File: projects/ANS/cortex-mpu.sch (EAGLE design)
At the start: 45 parts, among them IC1 LM1117MPX-3.3, U1 AT32UC3B164-AUT, Y1 7A-16

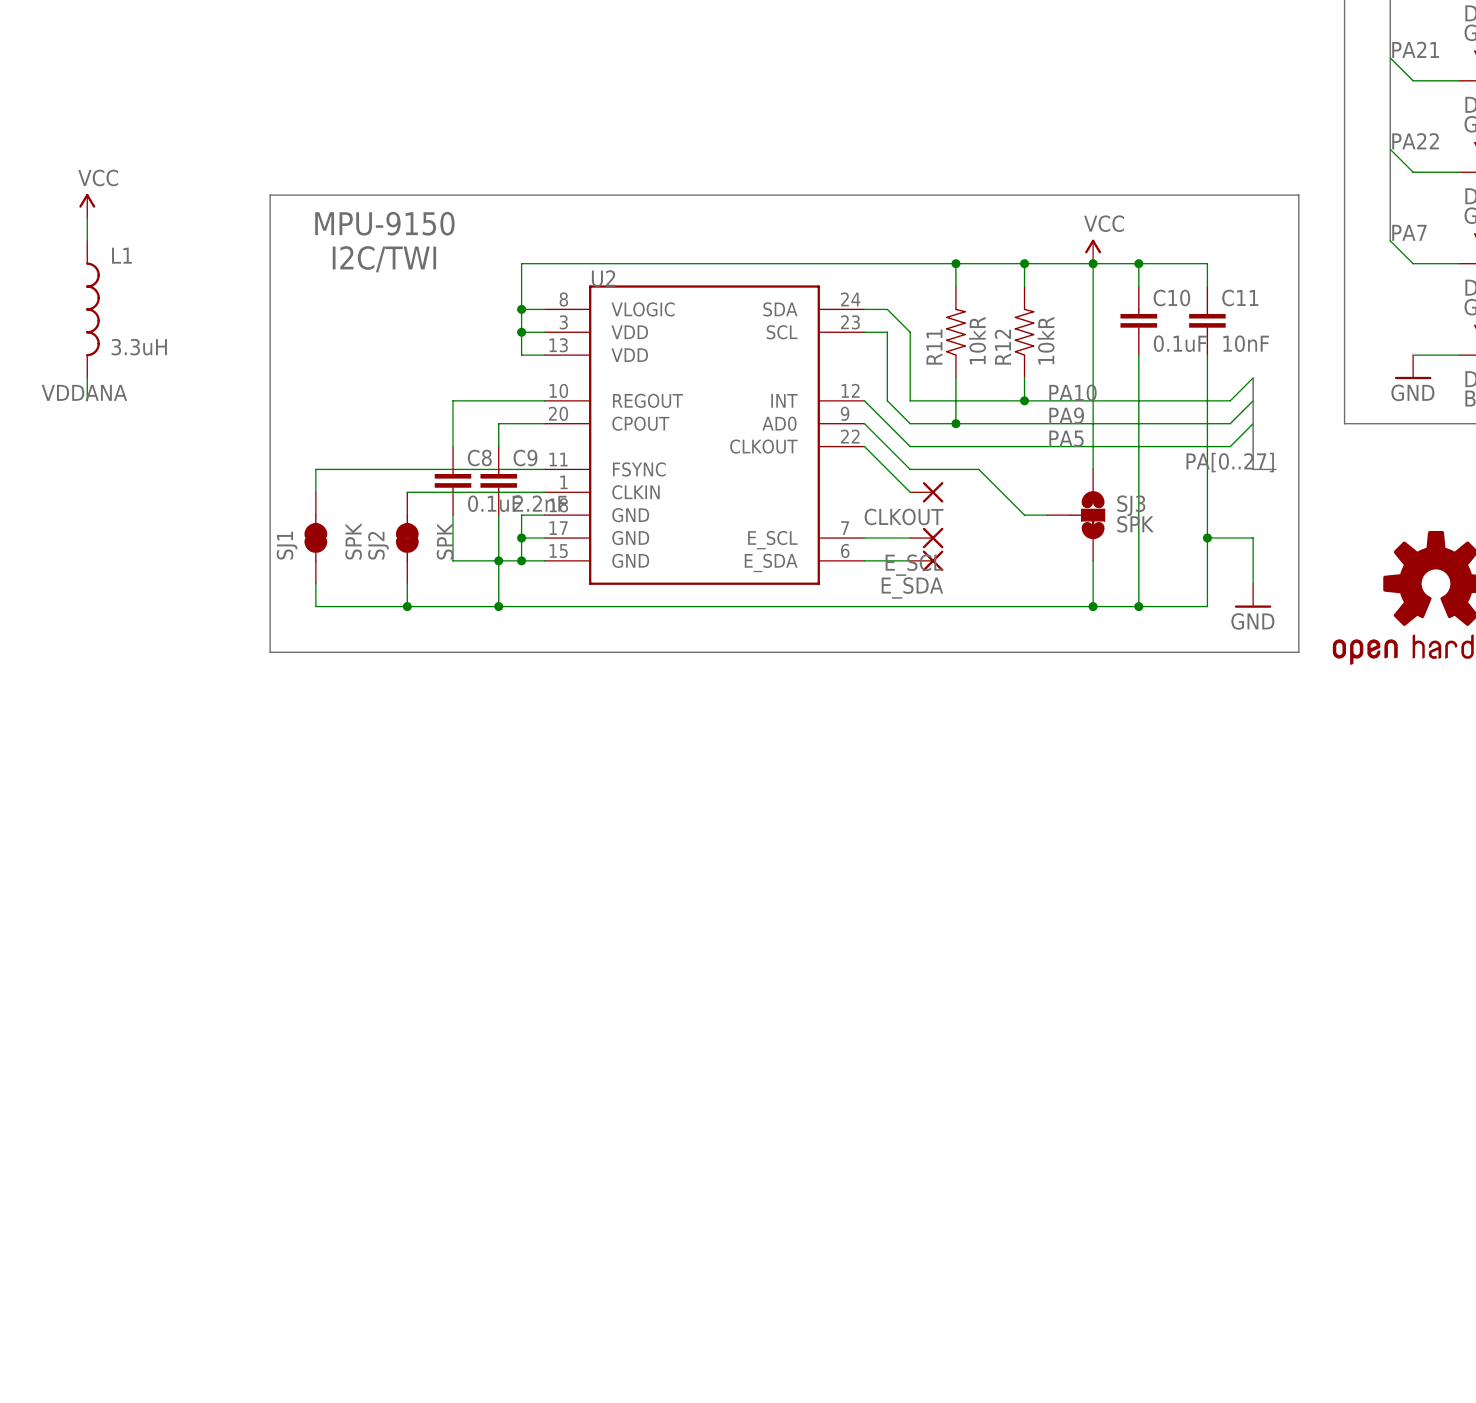
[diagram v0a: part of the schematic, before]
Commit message: Decoupling
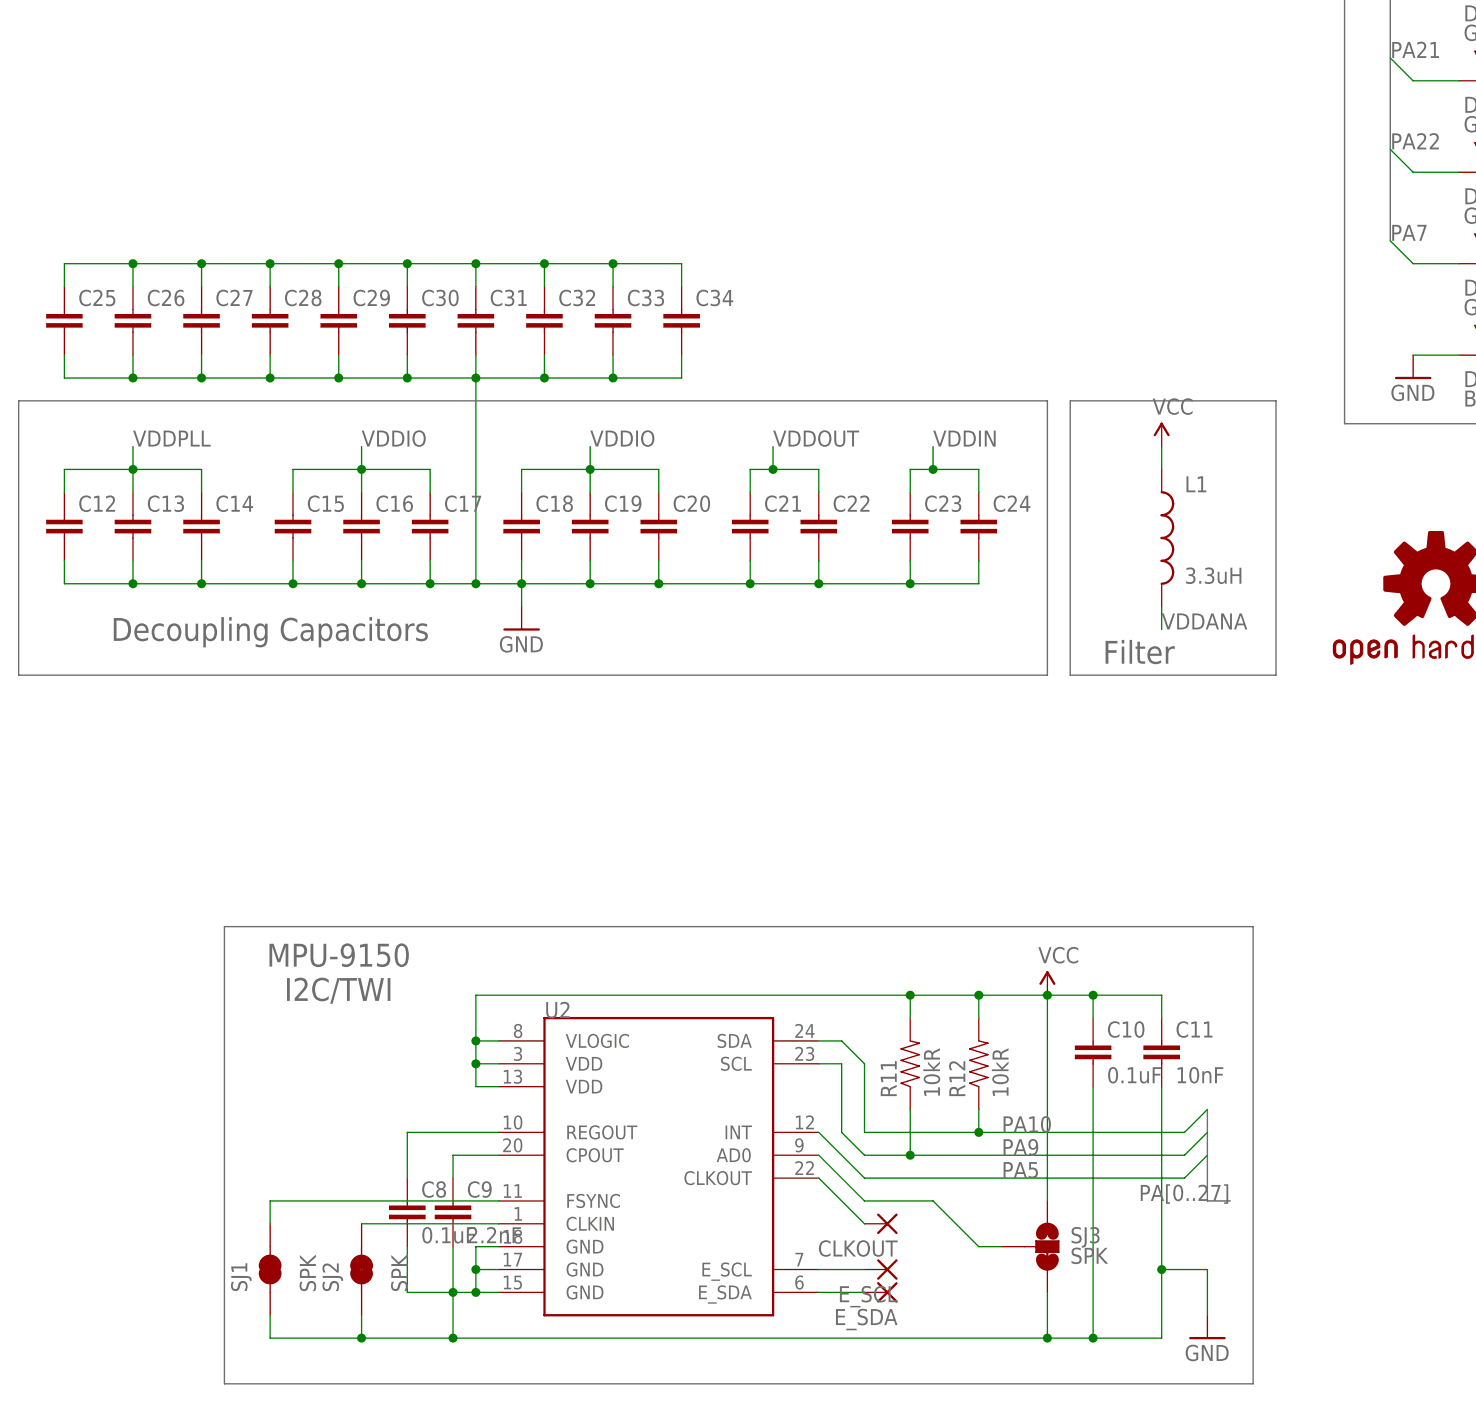
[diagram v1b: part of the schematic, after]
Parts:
- added C12, C13, C14, C15, C16, C17, C18, C19, C20, C21, C22, C23, C24, C25, C26, C27, C28, C29, C30, C31, C32, C33, C34: (no value), SparkFun-Passives:CAP0603-CAP
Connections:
- net GND: now also C12.2, C13.2, C14.2, C15.2, C16.2, C17.2, C18.2, C19.2, C20.2, C21.2, C22.2, C23.2, C24.2, C25.2, C26.2, C27.2, C28.2, C29.2, C30.2, C31.2, C32.2, C33.2, C34.2
- net VDDCORE: now also C25.1, C26.1, C27.1, C28.1, C29.1, C30.1, C31.1, C32.1, C33.1, C34.1
- net VDDIN: now also C23.1, C24.1
- net VDDIO: now also C15.1, C16.1, C17.1, C18.1, C19.1, C20.1
- net VDDOUT: now also C21.1, C22.1
- net VDDPLL: now also C12.1, C13.1, C14.1
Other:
- note added: "Decoupling Capacitors"
- note added: "Filter"
- moved on the sheet: C10, C11, C8, C9, CLKOUT, E_SCL, E_SDA, L1, R11, R12, SJ1, SJ2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

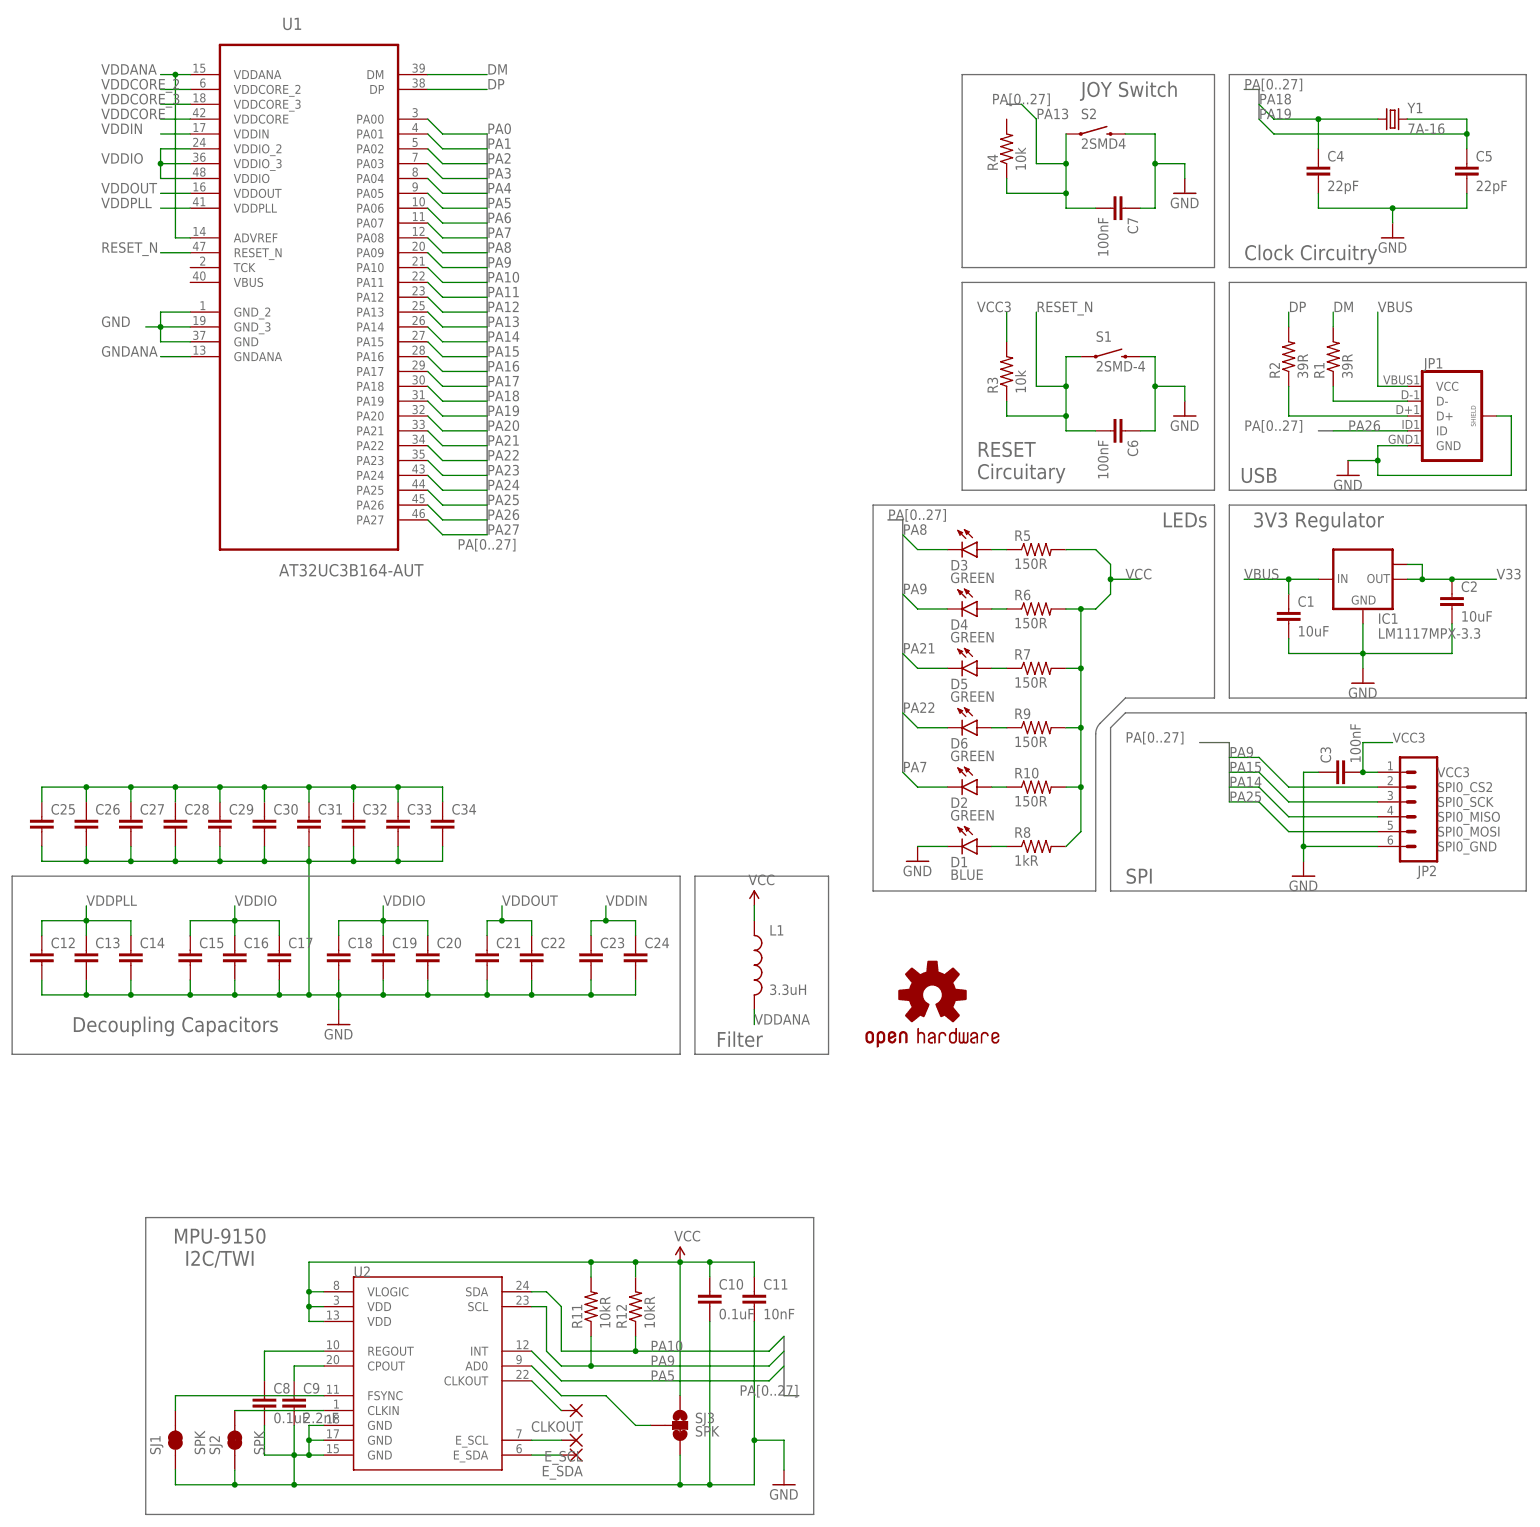
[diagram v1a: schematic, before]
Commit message: Decoupling Capr
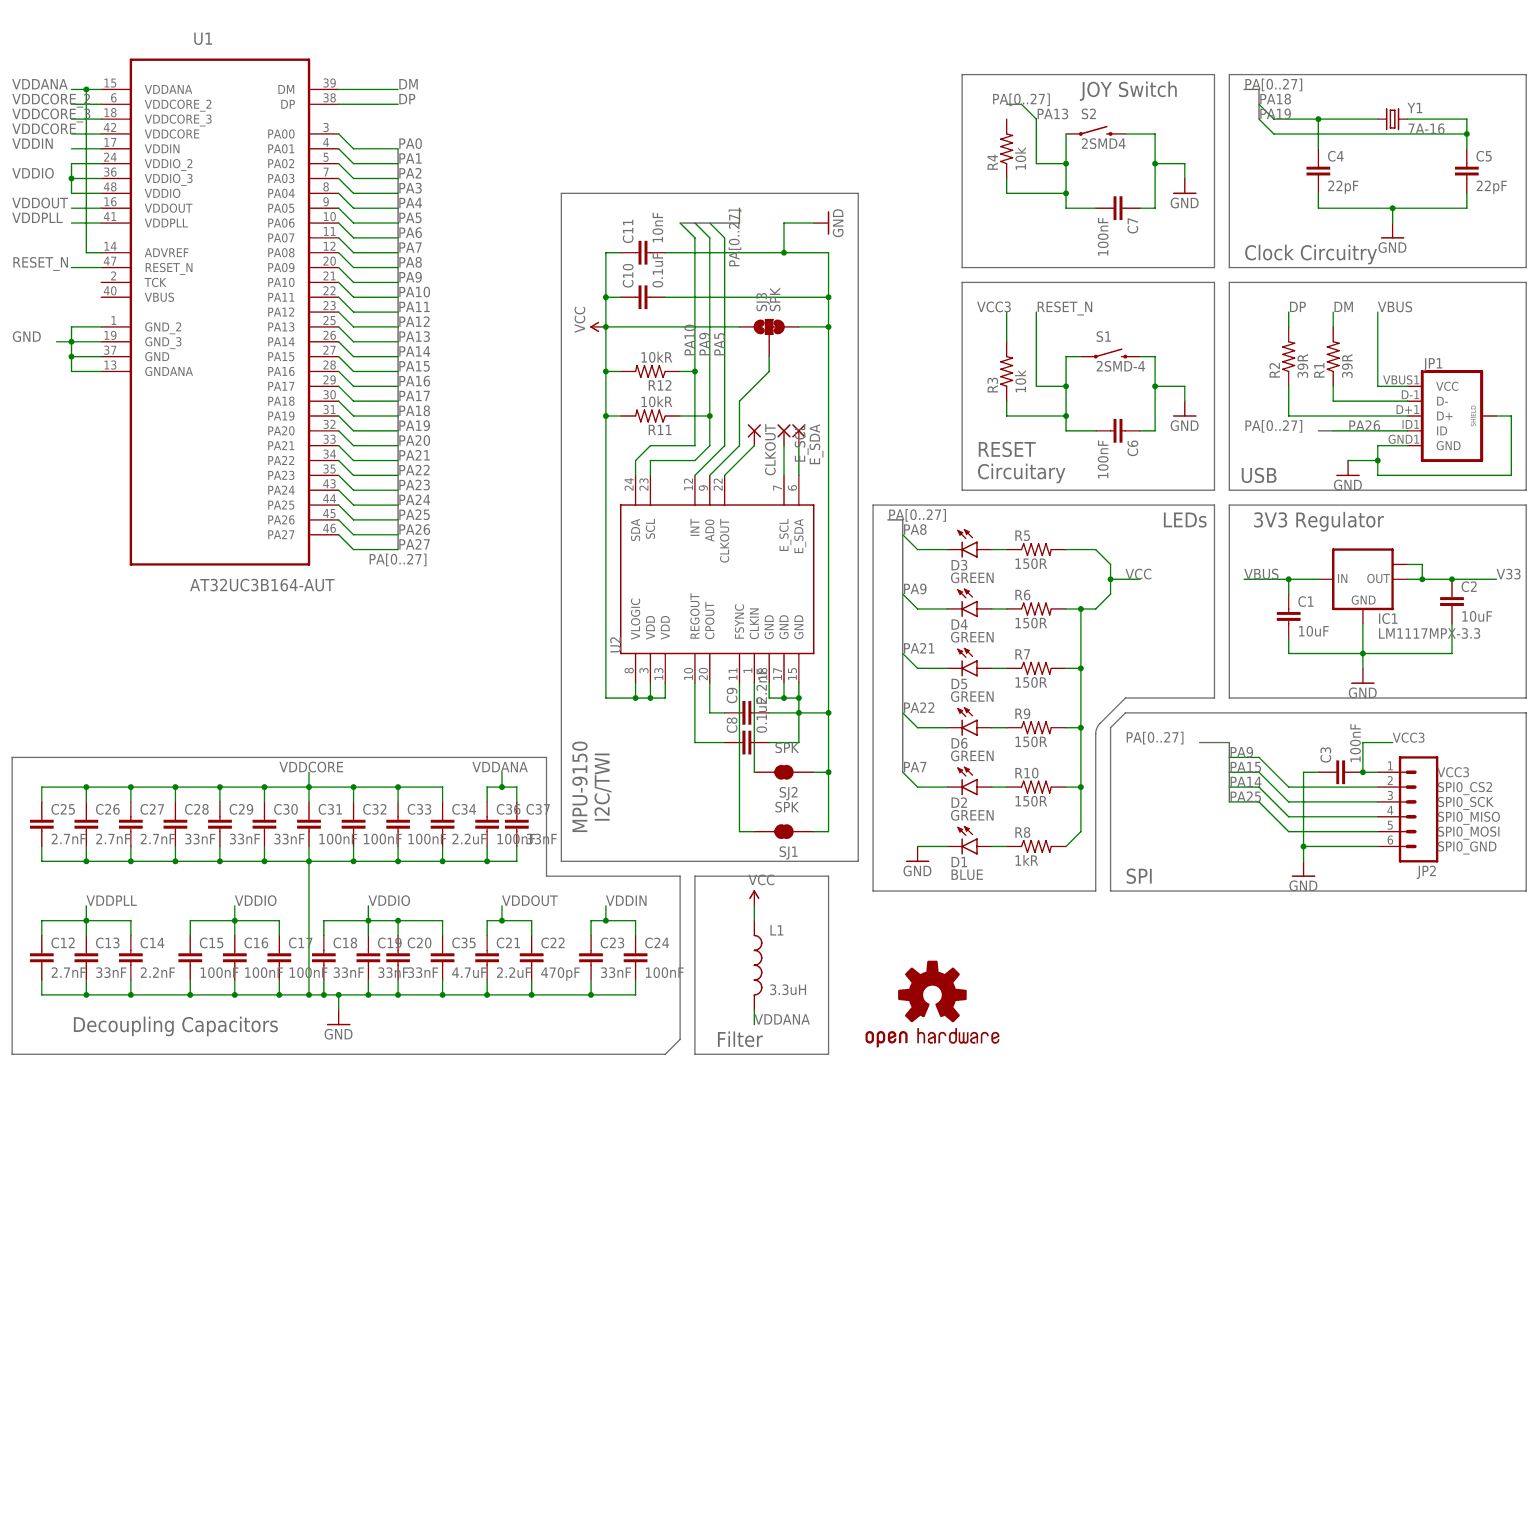
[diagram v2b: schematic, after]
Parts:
- added C35: 4.7uF, SparkFun-Passives:CAP0603-CAP
- added C36: 100nF, SparkFun-Passives:CAP0603-CAP
- added C37: 33nF, SparkFun-Passives:CAP0603-CAP
- C12, C25, C26, C27: value (none) -> 2.7nF
- C13, C18, C19, C20, C23, C28, C29, C30: value (none) -> 33nF
- C14: value (none) -> 2.2nF
- C15, C16, C17, C24, C31, C32, C33: value (none) -> 100nF
- C21, C34: value (none) -> 2.2uF
- C22: value (none) -> 470pF
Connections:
- removed net GNDANA: U1.GNDANA
- net GND: now also C35.2, C36.2, C37.2, U1.GNDANA
- net VDDANA: now also C36.1, C37.1
- net VDDIO: now also C35.1
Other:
- moved on the sheet: C10, C11, C18, C19, C20, C8, C9, CLKOUT, E_SCL, E_SDA, R11, R12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
